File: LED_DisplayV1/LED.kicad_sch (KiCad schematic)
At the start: 12 parts, among them U3 TPIC6C595N

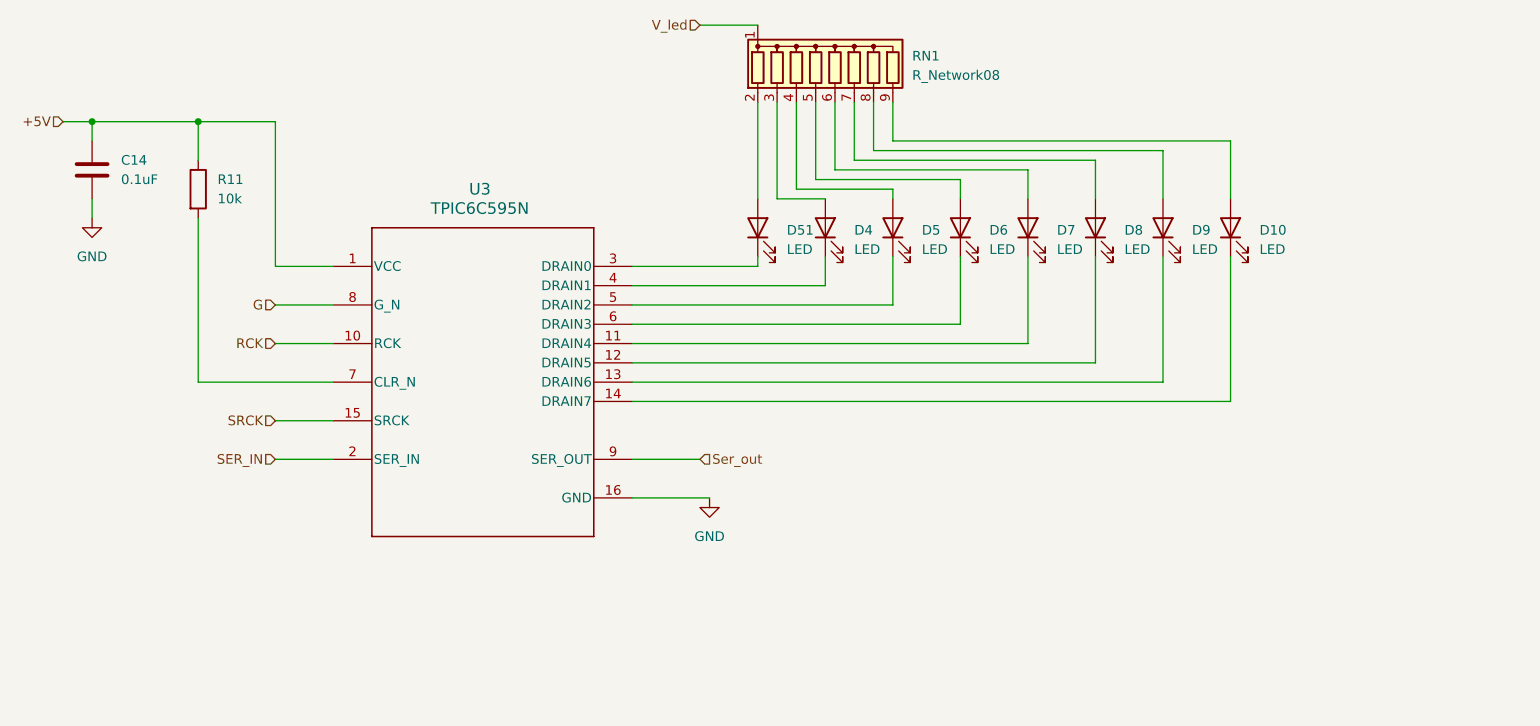
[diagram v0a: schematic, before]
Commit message: AddComponant
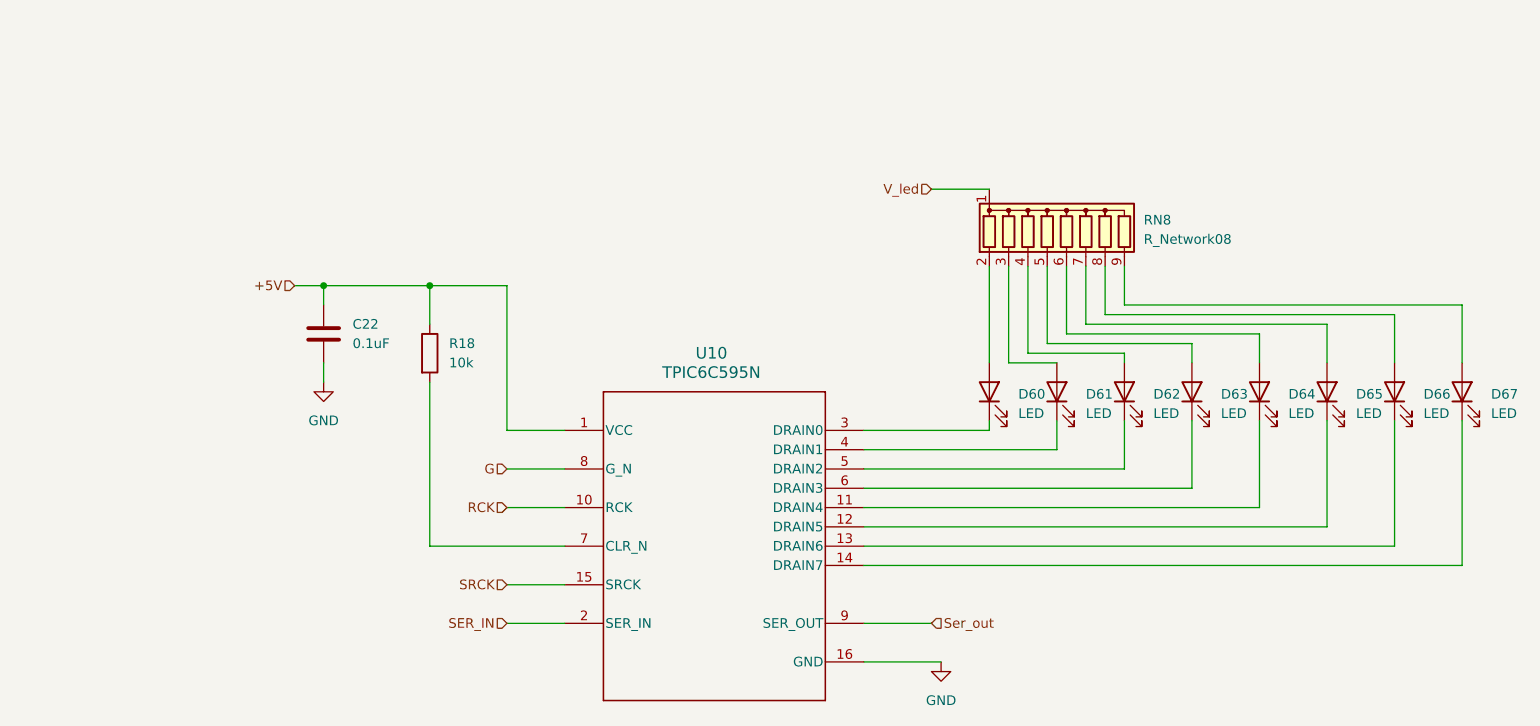
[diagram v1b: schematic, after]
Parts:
- removed C14: 0.1uF, Capacitor_SMD:C_0603_1608Metric_Pad1.08x0.95mm_HandSolder, symbol Device:C
- removed D10, D4, D5, D51, D6, D7, D8, D9: LED, symbol Device:LED
- removed R11: 10k, symbol Device:R
- removed RN1: R_Network08, Resistor_THT:R_Array_SIP9, symbol Device:R_Network08
- removed U3: TPIC6C595N, N0016A, symbol 2026-05-05_14-43-28:TPIC6C595N
- added C22: 0.1uF, Capacitor_SMD:C_0603_1608Metric_Pad1.08x0.95mm_HandSolder, symbol Device:C
- added D60, D61, D62, D63, D64, D65, D66, D67: LED, LED_THT:LED_Rectangular_W3.0mm_H2.0mm, symbol Device:LED
- added R18: 10k, Resistor_SMD:R_0402_1005Metric_Pad0.72x0.64mm_HandSolder, symbol Device:R
- added RN8: R_Network08, Resistor_THT:R_Array_SIP9, symbol Device:R_Network08
- added U10: TPIC6C595N, TPIC6C595N:N0016A, symbol 2026-05-05_14-43-28:TPIC6C595N
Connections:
- net +5V: now also C22.1, R18.1, U10.1 (VCC)
- net G: now also U10.8 (G_N)
- net GND: now also C22.2, U10.16 (GND)
- net RCK: now also U10.10 (RCK)
- net SER_IN: now also U10.2 (SER_IN)
- net SRCK: now also U10.15 (SRCK)
- net Ser_out: now also U10.9 (SER_OUT)
- net V_led: now also RN8.1 (common)
- new net: D60.1 (K), U10.3 (DRAIN0)
- new net: D60.2 (A), RN8.2 (R1)
- new net: D65.1 (K), U10.12 (DRAIN5)
- new net: D65.2 (A), RN8.7 (R6)
- new net: R18.2, U10.7 (CLR_N)
- new net: D61.1 (K), U10.4 (DRAIN1)
- new net: D61.2 (A), RN8.3 (R2)
- new net: D64.1 (K), U10.11 (DRAIN4)
- new net: D66.1 (K), U10.13 (DRAIN6)
- new net: D67.1 (K), U10.14 (DRAIN7)
- new net: D62.1 (K), U10.5 (DRAIN2)
- new net: D63.1 (K), U10.6 (DRAIN3)
- new net: D67.2 (A), RN8.9 (R8)
- new net: D62.2 (A), RN8.4 (R3)
- new net: D66.2 (A), RN8.8 (R7)
- new net: D63.2 (A), RN8.5 (R4)
- new net: D64.2 (A), RN8.6 (R5)
